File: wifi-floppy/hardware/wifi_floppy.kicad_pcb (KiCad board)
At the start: 2 copper layers, 96 x 62 mm, 13 parts, among them J1 FLOPPY34, J2 PWR-BERG, Q1 BSS138, Q2 BSS138, Q3 BSS138, Q4 BSS138, Q5 BSS138, Q6 BSS138, U1 Pico2W/PicoPlus2W, U2 74LVC541A

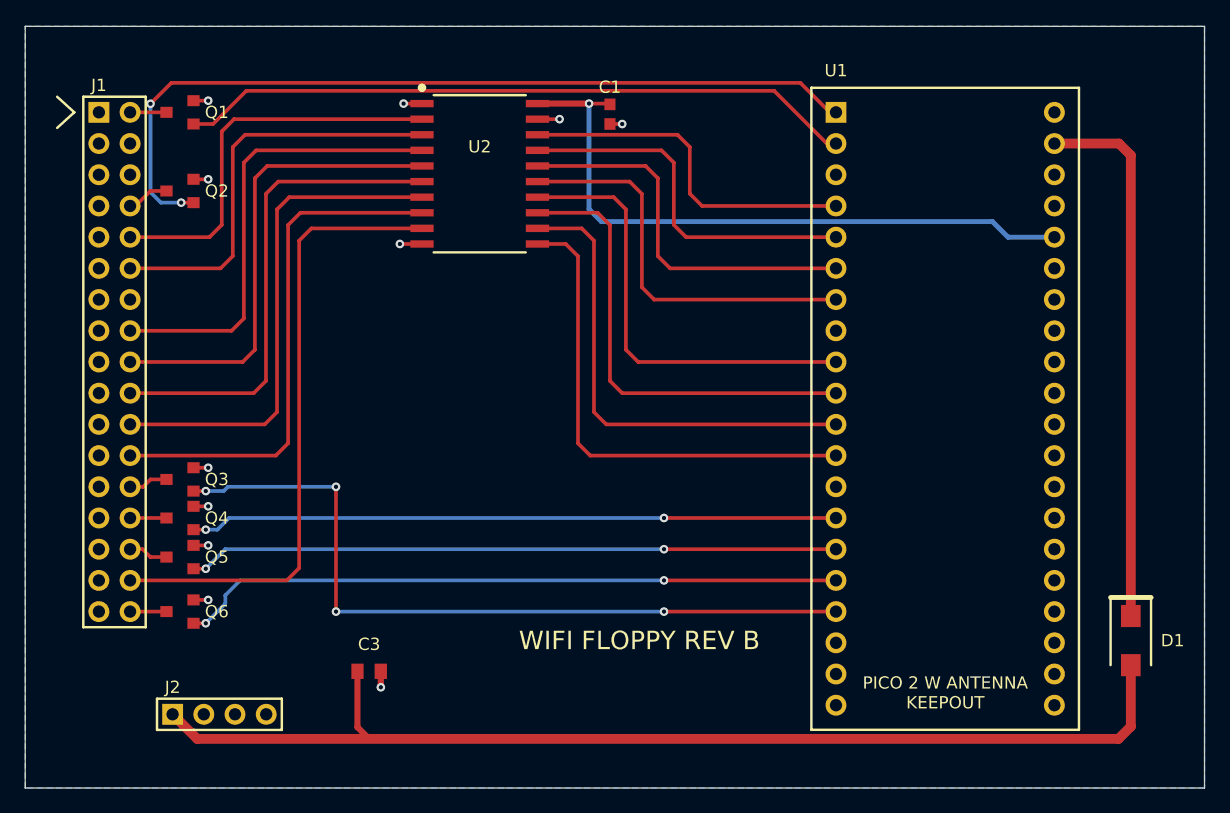
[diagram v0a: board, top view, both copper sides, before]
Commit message: [REV B] New PCB version.
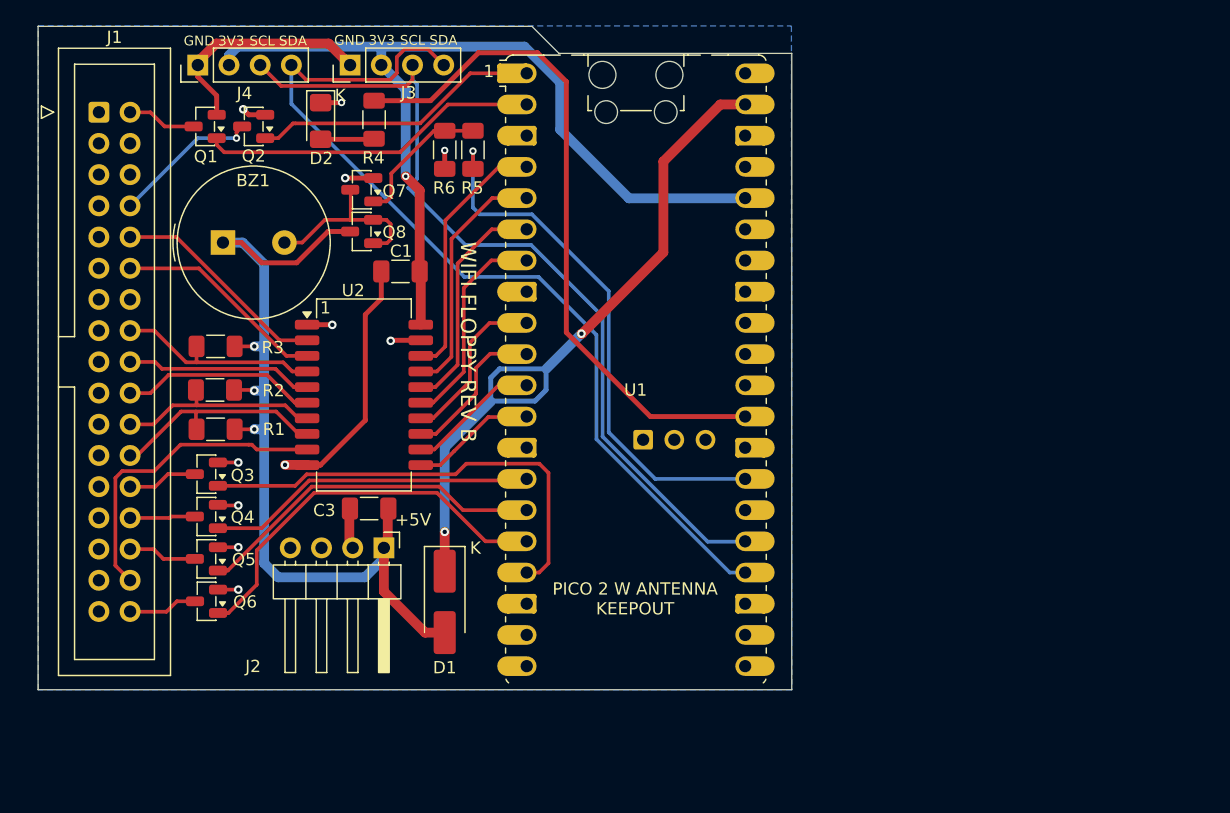
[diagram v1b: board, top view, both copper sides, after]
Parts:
- added BZ1: Buzzer, wifi-floppy-lib:Buzzer_TDK_PS1240P02BT_D12.2mm_H6.5mm, F.Cu at (116.1, 117.6)
- added D2: LED, wifi-floppy-lib:LED_1206_3216Metric_Pad1.42x1.75mm_HandSolder, F.Cu at (124.0, 107.7)
- added J3: Conn_01x04, wifi-floppy-lib:PinHeader_1x04_P2.54mm_Vertical, F.Cu at (126.5, 103.2)
- added J4: Conn_01x04, wifi-floppy-lib:PinHeader_1x04_P2.54mm_Vertical, F.Cu at (114.0, 103.2)
- added Q7: BSS138, wifi-floppy-lib:SOT-23, F.Cu at (127.4, 113.3)
- added Q8: BSS138, wifi-floppy-lib:SOT-23, F.Cu at (127.4, 116.7)
- added R1: 1k, wifi-floppy-lib:R_1206_3216Metric_Pad1.30x1.75mm_HandSolder, F.Cu at (115.5, 132.8)
- added R2: 1k, wifi-floppy-lib:R_1206_3216Metric_Pad1.30x1.75mm_HandSolder, F.Cu at (115.5, 129.6)
- added R3: 1k, wifi-floppy-lib:R_1206_3216Metric_Pad1.30x1.75mm_HandSolder, F.Cu at (115.5, 126.0)
- added R4: 1k, wifi-floppy-lib:R_1206_3216Metric_Pad1.30x1.75mm_HandSolder, F.Cu at (128.4, 107.6)
- added R5: 1k, wifi-floppy-lib:R_1206_3216Metric_Pad1.30x1.75mm_HandSolder, F.Cu at (136.4, 110.0)
- added R6: 10k, wifi-floppy-lib:R_1206_3216Metric_Pad1.30x1.75mm_HandSolder, F.Cu at (134.2, 110.0)
- C1: value 100n -> 100nF; footprint Capacitor_SMD:C_0603 -> wifi-floppy-lib:C_1206_3216Metric_Pad1.33x1.80mm_HandSolder
- C3: value 10u -> 10uF; footprint Capacitor_SMD:C_0805 -> wifi-floppy-lib:C_1206_3216Metric_Pad1.33x1.80mm_HandSolder
- D1: footprint Diode_SMD:D_SMA -> wifi-floppy-lib:D_SMA_Handsoldering
- J1: value FLOPPY34 -> Conn_02x17_Odd_Even; footprint Connector_PinHeader_2.54mm:PinHeader_2x17 -> wifi-floppy-lib:IDC-Header_2x17_P2.54mm_Vertical
- J2: value PWR-BERG -> Conn_01x04; footprint Connector_PinHeader_2.54mm:PinHeader_1x04 -> wifi-floppy-lib:PinHeader_1x04_P2.54mm_Horizontal
- Q1, Q2, Q3, Q4, Q5, Q6: footprint Package_TO_SOT_SMD:SOT-23 -> wifi-floppy-lib:SOT-23
- U1: value Pico2W/PicoPlus2W -> RaspberryPi_Pico_W; footprint wifi_floppy:Pico2W_THT -> wifi-floppy-lib:RaspberryPi_Pico_W_SMD_HandSolder
- U2: footprint Package_SO:SOIC-20W -> wifi-floppy-lib:SOIC-20W_7.5x15.4mm_P1.27mm
- moved D1 55.9 mm to (134.2, 146.8), turned to -90 degrees
- moved U1 26.5 mm to (149.7, 128.0)
- moved J2 21.9 mm to (129.2, 142.4), turned to -90 degrees
- moved C1 21.3 mm to (130.6, 120.0), turned to 180 degrees
- moved U2 20.3 mm to (127.6, 130.0)
- moved C3 13.2 mm to (128.0, 139.2), turned to 180 degrees
- moved Q2 7.97 mm to (118.6, 108.2), turned to 180 degrees
- moved Q1 2.35 mm to (114.7, 108.2), turned to 180 degrees
- moved Q6 2.32 mm to (114.8, 146.8), turned to 180 degrees
- moved Q3 2.19 mm to (114.8, 136.4), turned to 180 degrees
- moved Q5 2.16 mm to (114.8, 143.3), turned to 180 degrees
- moved Q4 2.15 mm to (114.8, 139.9), turned to 180 degrees
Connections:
- net +3V3 renamed +3.3V
- net VSYS renamed /VSYS
- J1 pad 14: (no net) -> unconnected-(J1-Pin_14-Pad14)
- J1 pad 4: (no net) -> unconnected-(J1-Pin_4-Pad4)
- J1 pad 6: (no net) -> unconnected-(J1-Pin_6-Pad6)
- J2 pad 4: +12V -> unconnected-(J2-Pin_4-Pad4)
- U1 pad 19: (no net) -> unconnected-(U1-GPIO14-Pad19)
- U1 pad 20: (no net) -> unconnected-(U1-GPIO15-Pad20)
- U1 pad 21: (no net) -> unconnected-(U1-GPIO16-Pad21)
- U1 pad 22: (no net) -> unconnected-(U1-GPIO17-Pad22)
- U1 pad 24: (no net) -> OLED_SDA
- U1 pad 25: (no net) -> OLED_SCL
- U1 pad 26: (no net) -> unconnected-(U1-GPIO20-Pad26)
- U1 pad 27: (no net) -> BUZZER
- U1 pad 29: (no net) -> ACT_LED
- U1 pad 30: (no net) -> unconnected-(U1-RUN-Pad30)
- U1 pad 31: (no net) -> unconnected-(U1-GPIO26_ADC0-Pad31)
- U1 pad 32: (no net) -> unconnected-(U1-GPIO27_ADC1-Pad32)
- U1 pad 34: (no net) -> unconnected-(U1-GPIO28_ADC2-Pad34)
- U1 pad 35: (no net) -> unconnected-(U1-ADC_VREF-Pad35)
- U1 pad 37: (no net) -> unconnected-(U1-3V3_EN-Pad37)
- U1 pad 40: (no net) -> unconnected-(U1-VBUS-Pad40)
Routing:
- net OLED_SDA: track 0.00 -> 76.1 mm
- net OLED_SCL: track 0.00 -> 70.1 mm
- net ACT_LED: track 0.00 -> 56.8 mm
- net GND: track 14.6 -> 61.4 mm
- net INDEX: track 68.6 -> 23.5 mm, vias 2 -> 0
- net BUZZER: track 0.00 -> 44.1 mm, vias 0 -> 1
- net SIDE: track 40.4 -> 9.51 mm
- net WGATE: track 39.1 -> 10.0 mm
- net CHNG: track 55.2 -> 27.6 mm
- net WPROT: track 52.7 -> 26.0 mm, vias 2 -> 0
- net WDATA: track 37.8 -> 11.8 mm
- net SIDE_B: track 51.2 -> 25.7 mm
- net RDATA: track 53.0 -> 28.0 mm, vias 2 -> 0
- net TRK0: track 62.6 -> 38.2 mm, vias 4 -> 0
- net WDATA_B: track 41.1 -> 16.8 mm
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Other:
- board size 96 x 62 mm -> 61.4 x 54 mm
- board text added: "+5V"
- board text added: "1"
- board text added: "3V3"
- board text added: "GND"
- board text added: "K"
- board text added: "SCL"
- board text added: "SDA"
